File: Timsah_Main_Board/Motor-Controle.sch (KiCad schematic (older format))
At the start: 9 parts, among them J10 SAĞ ARKA, J17 SOL ARKA, J18 SERVO Gripper, J19 SAĞ ÜST, J20 SOL ÜST, J3 SERVO Camera, J4 SAĞ ÖN, J9 SOL ÖN, U7 PCA9685PW

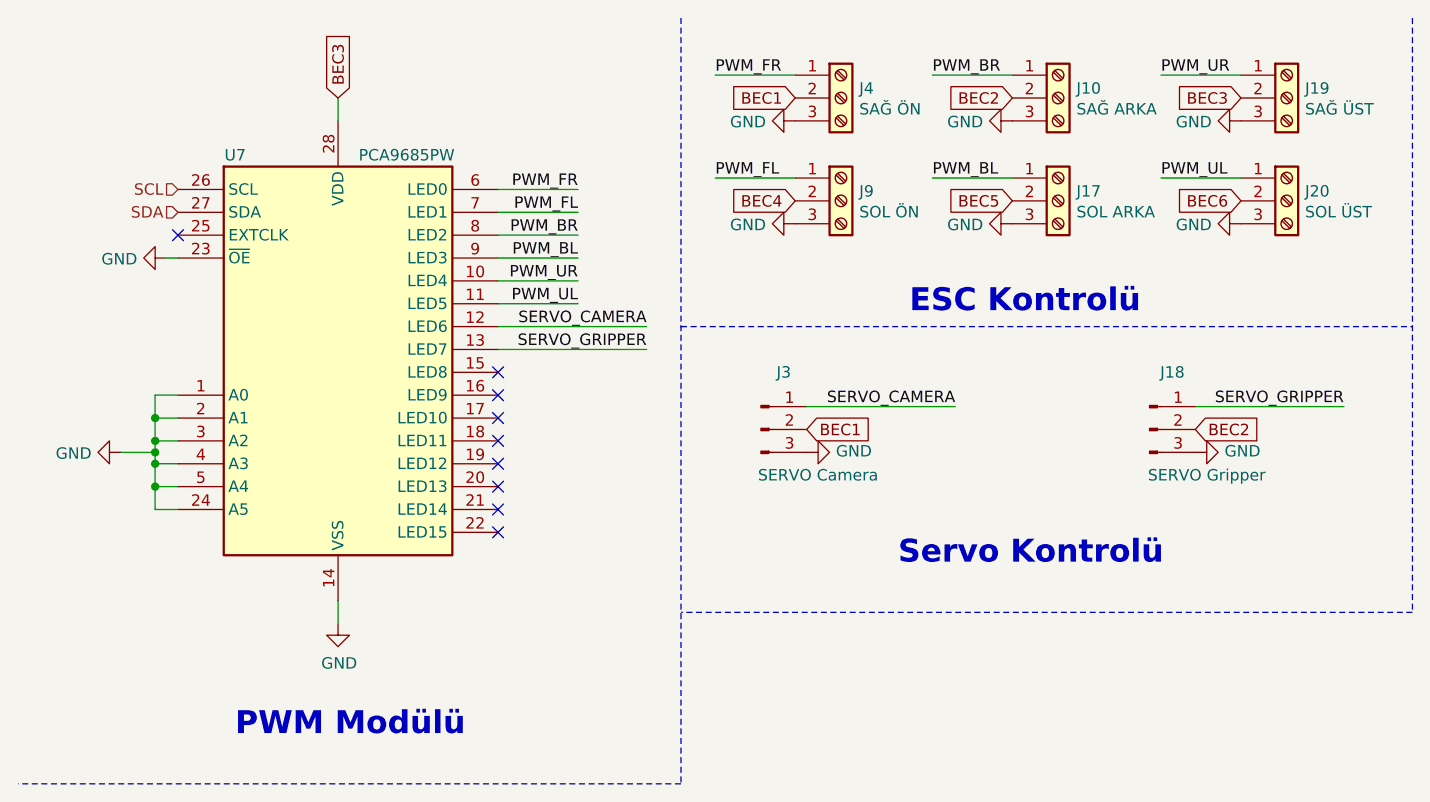
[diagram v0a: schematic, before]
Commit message: Schematic updates.
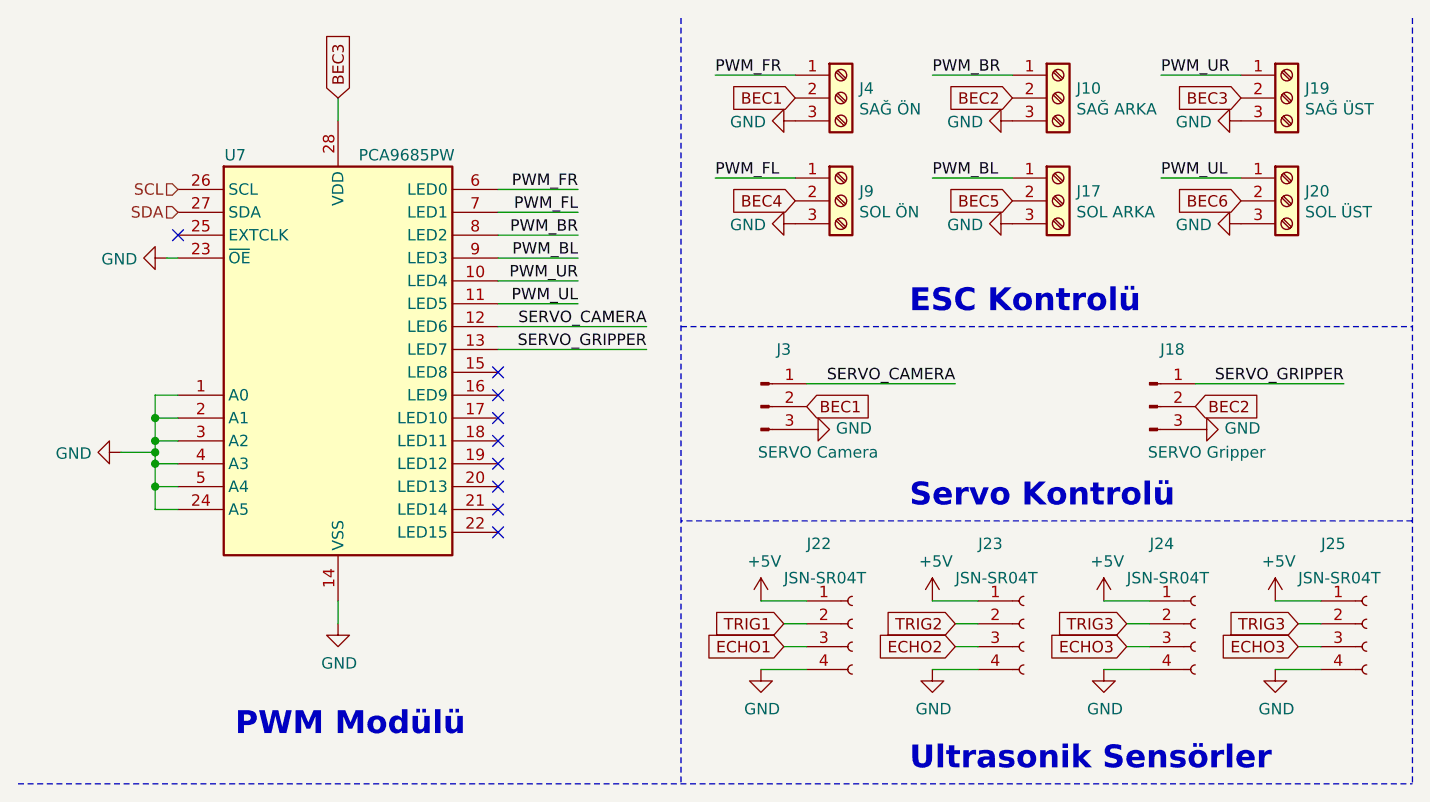
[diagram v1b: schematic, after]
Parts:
- added J22, J23, J24, J25: JSN-SR04T, symbol Connector:Conn_01x04_Female
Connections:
- net GND: now also J22.4 (Pin_4), J23.4 (Pin_4), J24.4 (Pin_4), J25.4 (Pin_4)
- new net +5V: J22.1 (Pin_1), J23.1 (Pin_1), J24.1 (Pin_1), J25.1 (Pin_1)
- new net ECHO1: J22.3 (Pin_3)
- new net ECHO2: J23.3 (Pin_3)
- new net ECHO3: J24.3 (Pin_3), J25.3 (Pin_3)
- new net TRIG1: J22.2 (Pin_2)
- new net TRIG2: J23.2 (Pin_2)
- new net TRIG3: J24.2 (Pin_2), J25.2 (Pin_2)
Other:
- note added: "Ultrasonik Sensörler"
- moved on the sheet: J18, J3

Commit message: Added software.
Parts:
- J18, J3: footprint (none) -> Connector_PinHeader_2.54mm:PinHeader_1x03_P2.54mm_Vertical
- J22, J23, J24, J25: footprint (none) -> Connector_PinHeader_2.54mm:PinHeader_1x04_P2.54mm_Vertical
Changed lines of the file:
@@
 F 0 "J3" H 3850 2450 50  0000 C CNN
 F 1 "SERVO Camera" H 4000 2000 50  0000 C CNN
-F 2 "" H 3750 2200 50  0001 C CNN
+F 2 "Connector_PinHeader_2.54mm:PinHeader_1x03_P2.54mm_Vertical" H 3750 2200 50  0001 C CNN
 F 3 "~" H 3750 2200 50  0001 C CNN
 	1    3750 2200
@@
 F 0 "J18" H 5550 2450 50  0000 C CNN
 F 1 "SERVO Gripper" H 5700 2000 50  0000 C CNN
-F 2 "" H 5450 2200 50  0001 C CNN
+F 2 "Connector_PinHeader_2.54mm:PinHeader_1x03_P2.54mm_Vertical" H 5450 2200 50  0001 C CNN
 F 3 "~" H 5450 2200 50  0001 C CNN
 	1    5450 2200
@@
 F 0 "J22" H 3950 3500 50  0000 L CNN
 F 1 "JSN-SR04T" H 3850 3350 50  0000 L CNN
-F 2 "" H 4150 3150 50  0001 C CNN
+F 2 "Connector_PinHeader_2.54mm:PinHeader_1x04_P2.54mm_Vertical" H 4150 3150 50  0001 C CNN
 F 3 "~" H 4150 3150 50  0001 C CNN
 	1    4150 3150
@@
 F 0 "J23" H 4700 3500 50  0000 L CNN
 F 1 "JSN-SR04T" H 4600 3350 50  0000 L CNN
-F 2 "" H 4900 3150 50  0001 C CNN
+F 2 "Connector_PinHeader_2.54mm:PinHeader_1x04_P2.54mm_Vertical" H 4900 3150 50  0001 C CNN
 F 3 "~" H 4900 3150 50  0001 C CNN
 	1    4900 3150
@@
 F 0 "J24" H 5450 3500 50  0000 L CNN
 F 1 "JSN-SR04T" H 5350 3350 50  0000 L CNN
-F 2 "" H 5650 3150 50  0001 C CNN
+F 2 "Connector_PinHeader_2.54mm:PinHeader_1x04_P2.54mm_Vertical" H 5650 3150 50  0001 C CNN
 F 3 "~" H 5650 3150 50  0001 C CNN
 	1    5650 3150
@@
 F 0 "J25" H 6200 3500 50  0000 L CNN
 F 1 "JSN-SR04T" H 6100 3350 50  0000 L CNN
-F 2 "" H 6400 3150 50  0001 C CNN
+F 2 "Connector_PinHeader_2.54mm:PinHeader_1x04_P2.54mm_Vertical" H 6400 3150 50  0001 C CNN
 F 3 "~" H 6400 3150 50  0001 C CNN
 	1    6400 3150
